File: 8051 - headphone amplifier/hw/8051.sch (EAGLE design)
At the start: 205 parts, among them IC1 317T, IC101 7805, IC102 CNY17, IC103 CNY17, IC104 CNY17, IC105 TSOP31236, IC106 ATMEGA328P-PU, IC107 CNY17, IC108 CNY17, IC109 CNY17, IC110 CNY17, IC111 CNY17, IC112 CNY17, IC113 CNY17, IC2 317T, IC3 7805, IC4L WM8816, IC4R WM8816, IC5L OPA132, IC5R OPA132, IC6L OPA132, IC6R OPA132, IC7 TPA6120, J1 DG301-2, J101 DG301-2, J102 M101, J103 M205, J104 M102, J105 M108, J106 M103, J2 DG301-2, J3 M103, J4 M101, J5L M103, J5R M103, J6 AMPHENOL ACJS-IH, J7 M102, M101 B40R, SW101 OMRON, SW102 ED1611S20, SW103 OMRON, T1 BS170, T2 IRF540, T3 IRF540, X101 8.00MHz

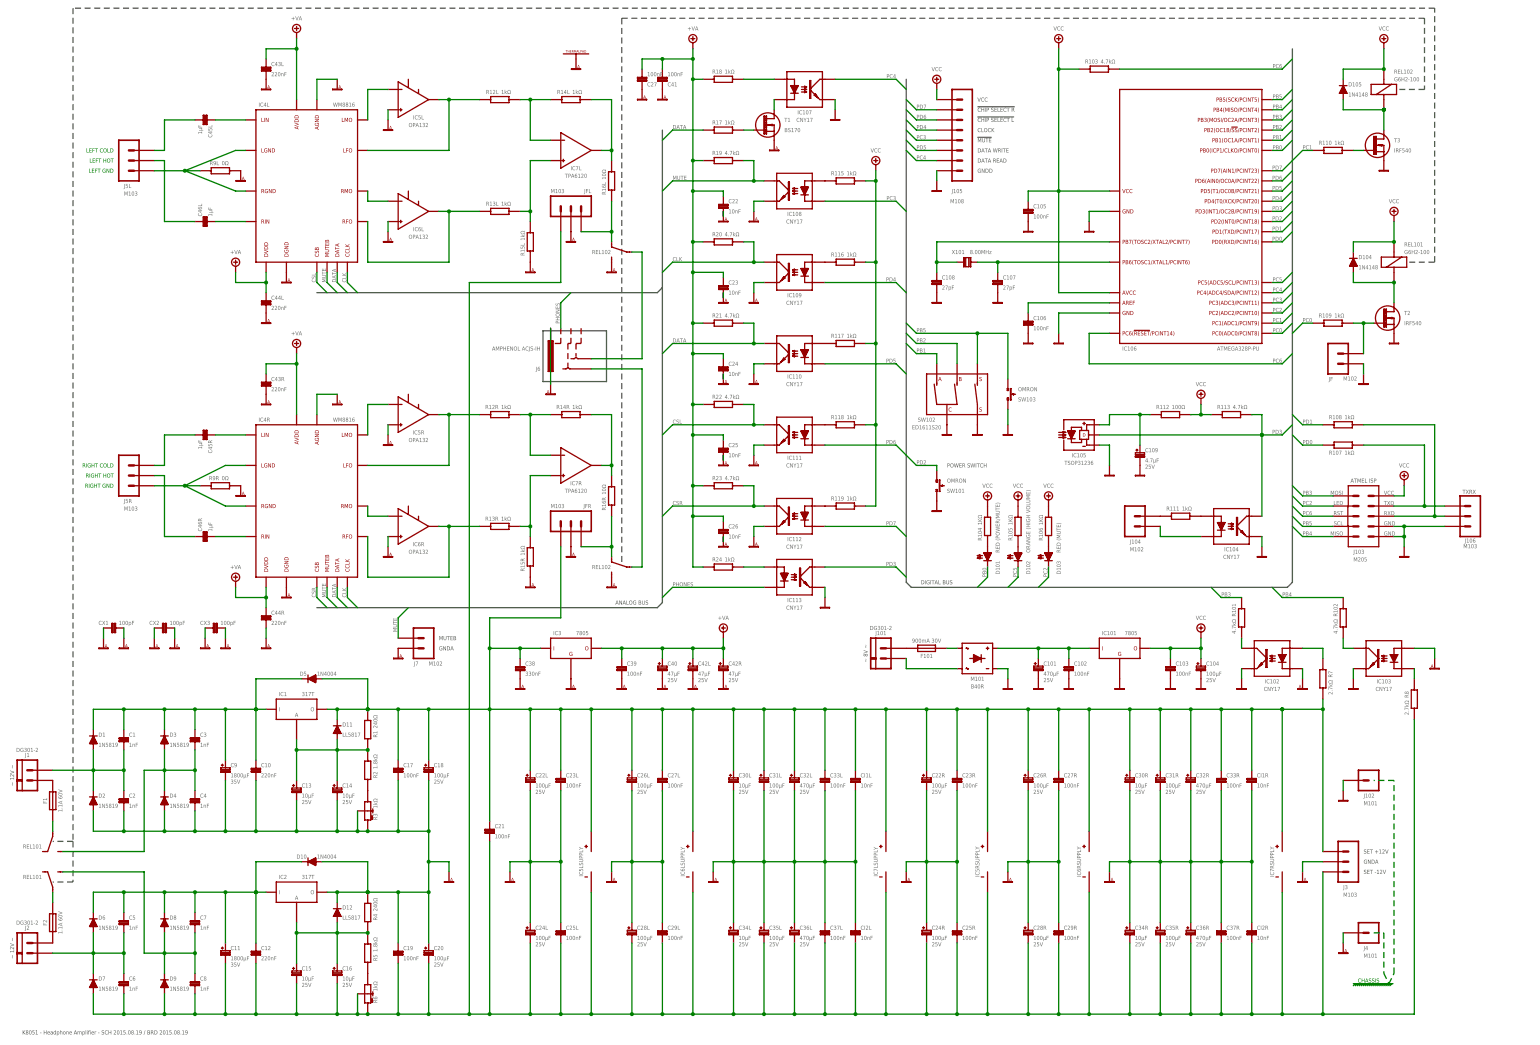
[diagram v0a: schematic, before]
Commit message: release
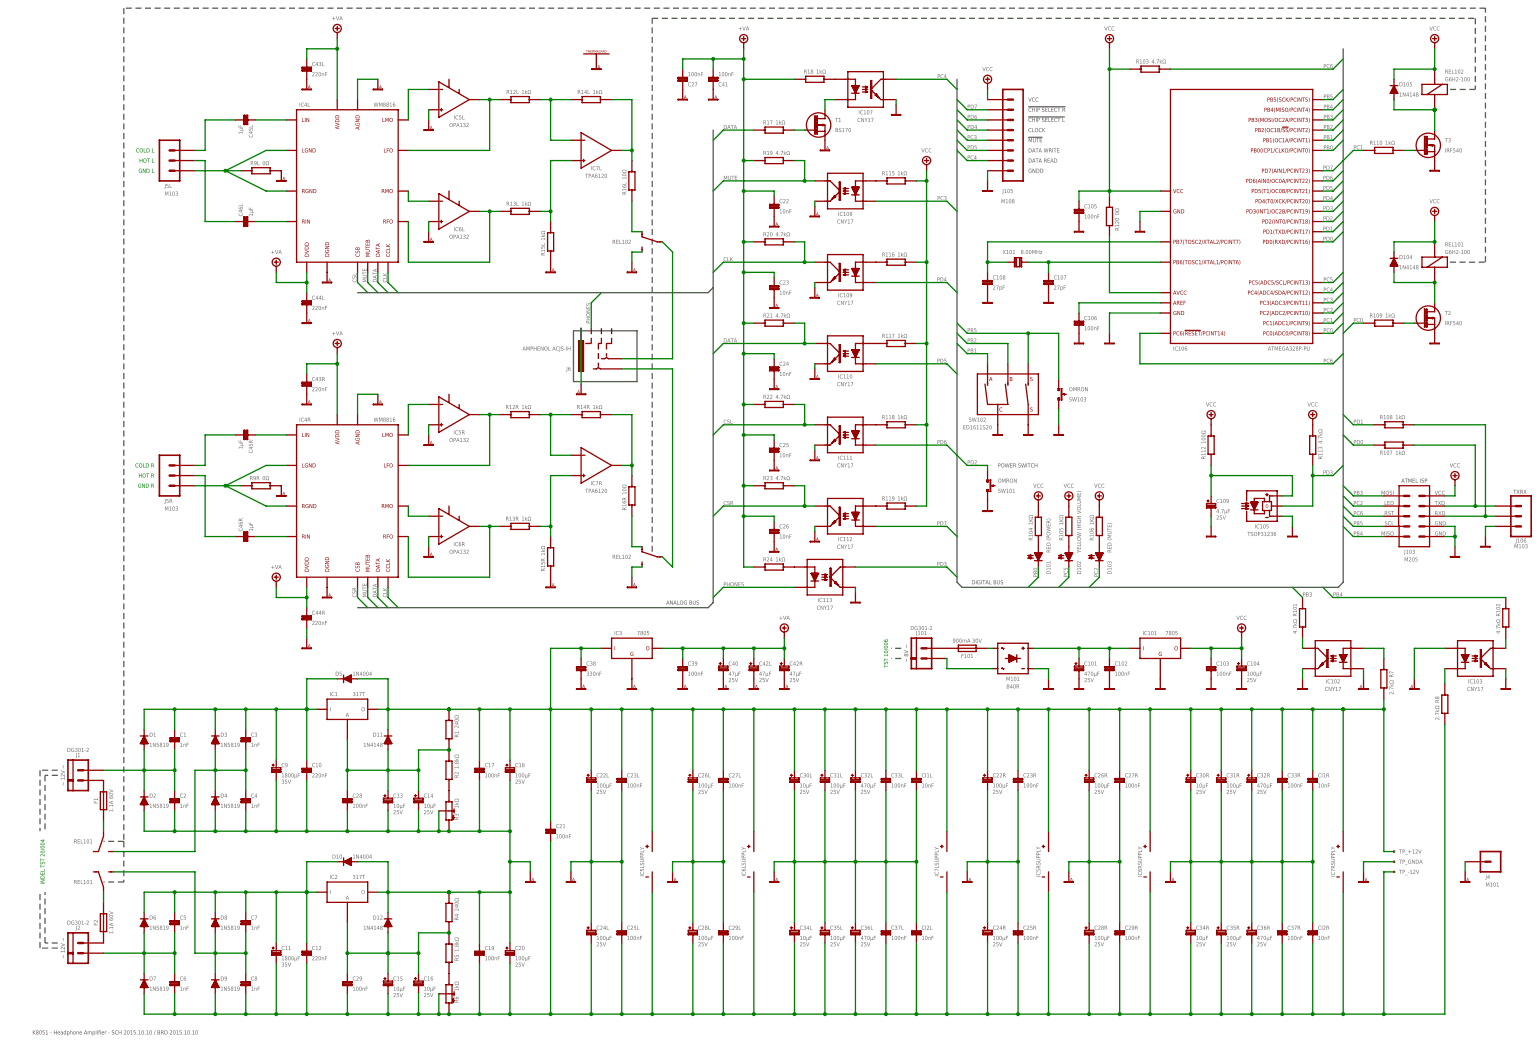
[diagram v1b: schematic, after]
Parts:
- removed CX1, CX2, CX3: 100pF, rcl:CC1206
- removed IC104: CNY17, optocoupler:CNY17F
- removed J102: M101, con-pins:1-1
- removed J104, J7, JF: M102, con-pins:1-2
- removed J3, JFL, JFR: M103, con-pins:1-3
- removed R111: 1kΩ, rcl:RR1206
- added C28, C29: 100nF, rcl:CC1812
- added R120: 0Ω, rcl:RR1206
- added TP_+12V, TP_-12V, TP_GNDA: TP, supply:TP
- D101: value RED (POWER/MUTE) -> RED (POWER)
- D102: value ORANGE (HIGH VOLUME) -> YELLOW (HIGH VOLUME)
- D11, D12: value LL5817 -> 1N4148; device diodes:DIODE-MELF-MLL41 -> diodes:1N4148DO35-7
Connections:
- net LH renamed AUDIOIN_LH
- net N$10 renamed TPAPOS_L
- net N$11 renamed RFO_L
- net N$12 renamed LFO_L
- net N$13 renamed AUDIOIN_LC
- net N$14 renamed TPANEG_L
- net N$16 renamed RIN_L
- net N$17 renamed TPAOUT_L
- net N$2 renamed AUDIOIN_LGND
- net N$20 renamed PHONES_L
- net N$22 renamed LIN_R
- net N$28 renamed RIN_R
- net N$29 renamed PHONES_R
- net N$3 renamed LMO_L
- net N$30 renamed RFO_R
- net N$34 renamed LFO_R
- net N$4 renamed RMO_L
- net N$41 renamed TPANEG_R
- net N$45 renamed AUDIOIN_RGND
- net N$46 renamed LMO_R
- net N$47 renamed RMO_R
- net N$5 renamed AUDIOIN_RC
- net N$51 renamed TPAPOS_R
- net N$7 renamed LIN_L
- net R3R renamed TPAOUT_R
- net RH renamed AUDIOIN_RH
- removed net N$19: JFR.1, R16R.1, REL1022.O
- removed net N$31: IC104.A, R111.2
- removed net N$37: JFL.1, R16L.1, REL1023.O
- removed net N$40: IC104.C, J104.2
- removed net N$42: J104.1, R111.1
- new net AVCC: IC106.AVCC, R120.1
- new net OUT_L: R16L.1, REL1023.O
- new net OUT_R: R16R.1, REL1022.O
- net GND: no longer IC104.EMIT, J102.1, JF.1
- net GNDA: now also C28.2, TP_GNDA.P$1; no longer CX1.1, CX1.2, CX2.1, CX2.2, CX3.1, CX3.2, J3.2, J7.2, JFL.2, JFR.2
- net MUTE: no longer J7.1
- net N$27: now also C28.1
- net N$60: no longer JF.2
- net N$8: now also C29.1
- net PD3: no longer IC104.COL
- net V+: now also TP_+12V.P$1; no longer J3.1, JFR.3
- net V-: now also C29.2, TP_-12V.P$1; no longer J3.3, JFL.3
- net VCC: now also R120.2; no longer IC106.AVCC
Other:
- note added: "COLD L HOT L GND L"
- note added: "COLD R HOT R GND R"
- note added: "INDEL TST 20/004"
- note added: "K8051 - Headphone Amplifier - SCH 2015.10.10 / BRD 2015.10.10"
- note added: "TST 10/006"
- note removed: "CHASSIS"
- note removed: "K8051 - Headphone Amplifier - SCH 2015.08.19 / BRD 2015.08.19"
- note removed: "LEFT COLD LEFT HOT LEFT GND"
- note removed: "MUTEB GNDA"
- note removed: "RIGHT COLD RIGHT HOT RIGHT GND"
- note removed: "SET +12V GNDA SET -12V"
- moved on the sheet: C1, C10, C101, C102, C103, C104, C105, C106, C107, C108, C109, C11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
